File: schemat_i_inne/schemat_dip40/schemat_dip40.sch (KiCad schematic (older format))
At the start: 5 parts, among them J1 Conn_01x06_Female, U1 ATmega32A-PU, U2 Wincom_WG12864D-SFYLY, U3 SD_card_reader

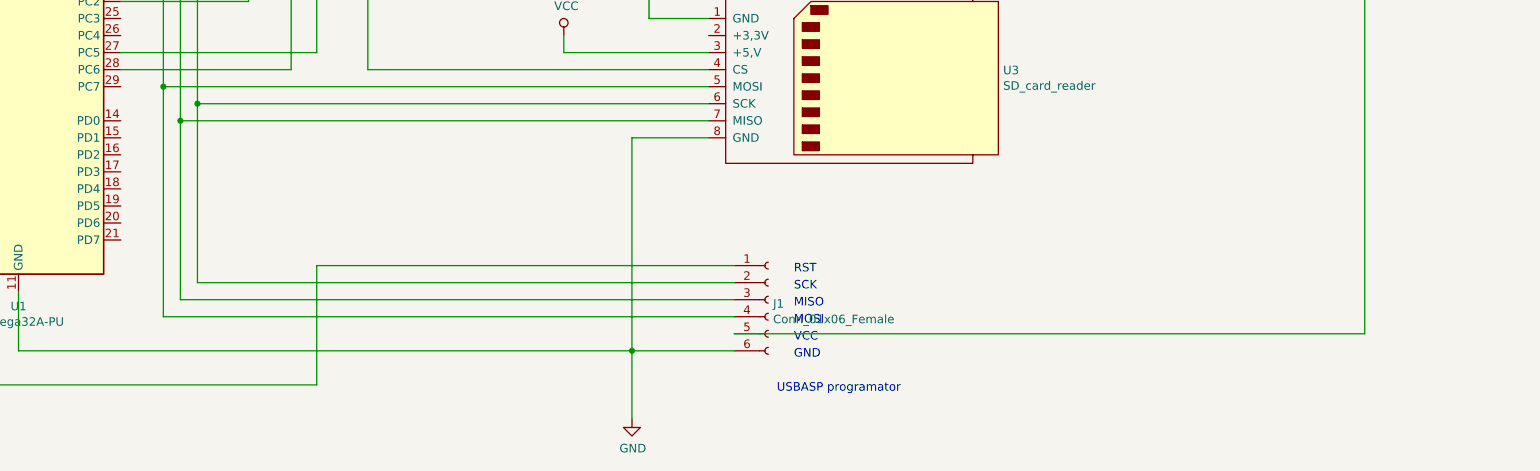
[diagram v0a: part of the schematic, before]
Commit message: Spaghetti dodane
Dodano przyciski do spaghetti układu
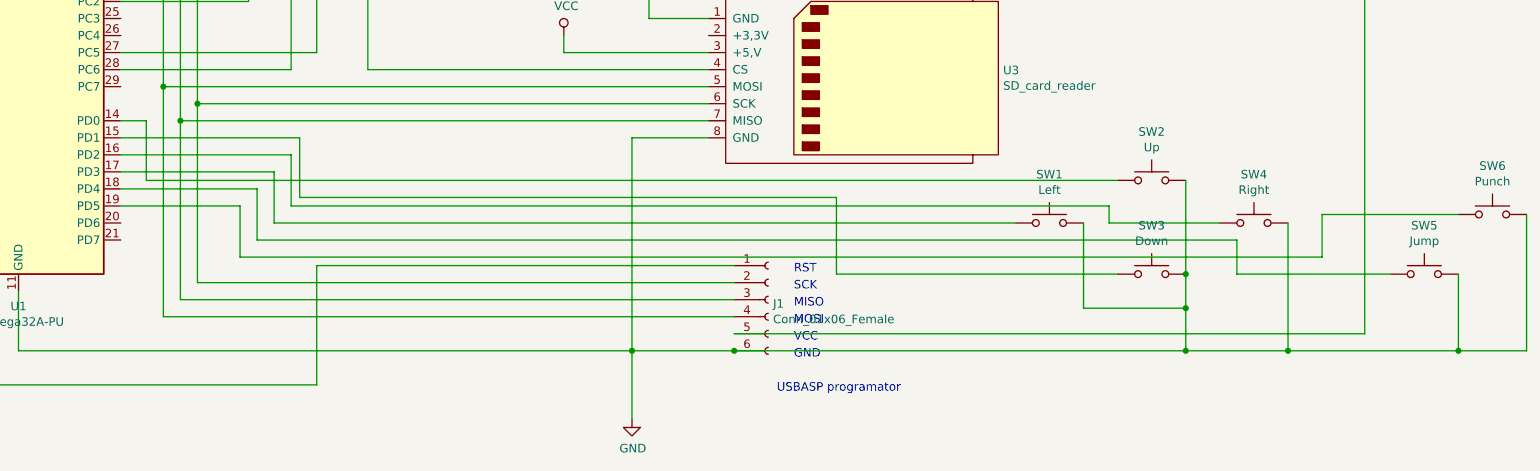
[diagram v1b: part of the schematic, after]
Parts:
- added SW1: Left, symbol Switch:SW_Push
- added SW2: Up, symbol Switch:SW_Push
- added SW3: Down, symbol Switch:SW_Push
- added SW4: Right, symbol Switch:SW_Push
- added SW5: Jump, symbol Switch:SW_Push
- added SW6: Punch, symbol Switch:SW_Push
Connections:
- net GND: now also SW1.2, SW2.2, SW3.2, SW4.2, SW5.2, SW6.2
- net at U1.14 (PD0): now also SW2.1
- net at U1.15 (PD1): now also SW3.1
- net at U1.16 (PD2): now also SW4.1
- net at U1.17 (PD3): now also SW1.1
- net at U1.18 (PD4): now also SW5.1
- net at U1.19 (PD5): now also SW6.1
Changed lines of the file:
@@
 $EndDescr
-$Comp
-L MCU_Microchip_ATmega:ATmega32A-PU U1
-U 1 1 61D4C9CD
-P 2250 3250
-F 0 "U1" H 2250 1161 50  0000 C CNN
-F 1 "ATmega32A-PU" H 2250 1070 50  0000 C CNN
-F 2 "Package_DIP:DIP-40_W15.24mm" H 2250 3250 50  0001 C CIN
-F 3 "http://ww1.microchip.com/downloads/en/DeviceDoc/atmel-8155-8-bit-microcontroller-avr-atmega32a_datasheet.pdf" H 2250 3250 50  0001 C CNN
-	1    2250 3250
-	1    0    0    -1
-$EndComp
 $Comp
 L schemat_dip40-rescue:Wincom_WG12864D-SFYLY-Display_Graphic U2
@@
 	5550 2150 5550 1550
 Wire Wire Line
-	5550 1550 2850 1550
-Wire Wire Line
 	6100 2250 5450 2250
 Wire Wire Line
 	5450 2250 5450 1650
 Wire Wire Line
-	5450 1650 2850 1650
-Wire Wire Line
 	6100 2350 5350 2350
 Wire Wire Line
 	5350 2350 5350 1750
 Wire Wire Line
-	5350 1750 2850 1750
-Wire Wire Line
 	6100 2450 5250 2450
 Wire Wire Line
 	5250 2450 5250 1850
 Wire Wire Line
-	5250 1850 2850 1850
-Wire Wire Line
 	6100 2550 5150 2550
 Wire Wire Line
 	5150 2550 5150 1950
 Wire Wire Line
-	5150 1950 2850 1950
-Wire Wire Line
 	6100 2650 5050 2650
 Wire Wire Line
 	5050 2650 5050 2050
 Wire Wire Line
-	5050 2050 2850 2050
-Wire Wire Line
 	6100 2750 4950 2750
 Wire Wire Line
 	4950 2750 4950 2150
 Wire Wire Line
-	4950 2150 2850 2150
-Wire Wire Line
 	6100 2850 4850 2850
 Wire Wire Line
 	4850 2850 4850 2250
 Wire Wire Line
-	4850 2250 2850 2250
-Wire Wire Line
 	6100 1650 5950 1650
 Wire Wire Line
@@
 	3500 1200 3500 3350
 Wire Wire Line
-	3500 3350 2850 3350
-Wire Wire Line
 	6100 1750 5850 1750
 Wire Wire Line
@@
 Wire Wire Line
 	3600 1300 3600 3550
-Wire Wire Line
-	3600 3550 2850 3550
 $Comp
 L power:VCC #PWR04
@@
 	3700 1450 3700 3450
 Wire Wire Line
-	3700 3450 2850 3450
-Wire Wire Line
 	6600 3050 6600 3200
 Wire Wire Line
@@
 	3850 3300 3850 3950
 Wire Wire Line
-	3850 3950 2850 3950
-Wire Wire Line
 	7100 2850 7400 2850
 Wire Wire Line
@@
 Wire Wire Line
 	4000 3400 4000 3850
-Wire Wire Line
-	4000 3850 2850 3850
 Wire Wire Line
 	7100 2350 7600 2350
@@
 $EndComp
 Wire Wire Line
-	2250 1250 2250 900
-Wire Wire Line
-	2350 1250 2350 900
-Wire Wire Line
 	2350 900  2250 900
 Connection ~ 2250 900
-Wire Wire Line
-	2250 5250 2250 5600
 Wire Wire Line
 	2250 5600 5850 5600
@@
 	1350 5800 1350 1550
 Wire Wire Line
-	1350 1550 1650 1550
-Wire Wire Line
 	6450 5200 3300 5200
 Wire Wire Line
 	3300 5200 3300 4150
 Wire Wire Line
-	3300 3150 2850 3150
-Wire Wire Line
 	6450 5300 3200 5300
 Wire Wire Line
 	3200 5300 3200 4250
 Wire Wire Line
-	3200 3050 2850 3050
-Wire Wire Line
 	6450 5400 3100 5400
 Wire Wire Line
 	3100 5400 3100 4050
 Wire Wire Line
-	3100 2950 2850 2950
-Wire Wire Line
 	6300 3950 4300 3950
 Wire Wire Line
 	4300 3950 4300 2650
-Wire Wire Line
-	4300 2650 2850 2650
 Wire Wire Line
 	6300 4050 3100 4050
@@
 	10150 5500 10150 2550
 Connection ~ 10150 2550
+$Comp
+L Switch:SW_Push SW2
+U 1 1 6261EEBB
+P 8900 4600
+F 0 "SW2" H 8900 4885 50  0000 C CNN
+F 1 "Up" H 8900 4794 50  0000 C CNN
+F 2 "" H 8900 4800 50  0001 C CNN
+F 3 "~" H 8900 4800 50  0001 C CNN
+	1    8900 4600
+	1    0    0    -1
+$EndComp
+$Comp
+L Switch:SW_Push SW3
+U 1 1 6261FEC3
+P 8900 5150
+F 0 "SW3" H 8900 5435 50  0000 C CNN
+F 1 "Down" H 8900 5344 50  0000 C CNN
+F 2 "" H 8900 5350 50  0001 C CNN
+F 3 "~" H 8900 5350 50  0001 C CNN
+	1    8900 5150
+	1    0    0    -1
+$EndComp
+$Comp
+L Switch:SW_Push SW4
+U 1 1 6262059D
+P 9500 4850
+F 0 "SW4" H 9500 5135 50  0000 C CNN
+F 1 "Right" H 9500 5044 50  0000 C CNN
+F 2 "" H 9500 5050 50  0001 C CNN
+F 3 "~" H 9500 5050 50  0001 C CNN
+	1    9500 4850
+	1    0    0    -1
+$EndComp
+$Comp
+L Switch:SW_Push SW1
+U 1 1 62620D64
+P 8300 4850
+F 0 "SW1" H 8300 5135 50  0000 C CNN
+F 1 "Left" H 8300 5044 50  0000 C CNN
+F 2 "" H 8300 5050 50  0001 C CNN
+F 3 "~" H 8300 5050 50  0001 C CNN
+	1    8300 4850
+	1    0    0    -1
+$EndComp
+$Comp
+L Switch:SW_Push SW5
+U 1 1 626213AA
+P 10500 5150
+F 0 "SW5" H 10500 5435 50  0000 C CNN
+F 1 "Jump" H 10500 5344 50  0000 C CNN
+F 2 "" H 10500 5350 50  0001 C CNN
+F 3 "~" H 10500 5350 50  0001 C CNN
+	1    10500 5150
+	1    0    0    -1
+$EndComp
+$Comp
+L Switch:SW_Push SW6
+U 1 1 6262299A
+P 10900 4800
+F 0 "SW6" H 10900 5085 50  0000 C CNN
+F 1 "Punch" H 10900 4994 50  0000 C CNN
+F 2 "" H 10900 5000 50  0001 C CNN
+F 3 "~" H 10900 5000 50  0001 C CNN
+	1    10900 4800
+	1    0    0    -1
+$EndComp
+Wire Wire Line
+	1350 1550 1650 1550
+Wire Wire Line
+	3300 3150 2850 3150
+Wire Wire Line
+	3200 3050 2850 3050
+Wire Wire Line
+	3100 2950 2850 2950
+Wire Wire Line
+	5550 1550 2850 1550
+Wire Wire Line
+	5450 1650 2850 1650
+Wire Wire Line
+	5350 1750 2850 1750
+Wire Wire Line
+	5250 1850 2850 1850
+Wire Wire Line
+	5150 1950 2850 1950
+Wire Wire Line
+	5050 2050 2850 2050
+Wire Wire Line
+	4950 2150 2850 2150
+Wire Wire Line
+	4850 2250 2850 2250
+Wire Wire Line
+	2350 1250 2350 900
+Wire Wire Line
+	4300 2650 2850 2650
+Wire Wire Line
+	3850 3950 2850 3950
+Wire Wire Line
+	4000 3850 2850 3850
+Wire Wire Line
+	3600 3550 2850 3550
+Wire Wire Line
+	3700 3450 2850 3450
+Wire Wire Line
+	3500 3350 2850 3350
+Wire Wire Line
+	2250 5250 2250 5600
+Wire Wire Line
+	2250 1250 2250 900
+$Comp
+L MCU_Microchip_ATmega:ATmega32A-PU U1
+U 1 1 61D4C9CD
+P 2250 3250
+F 0 "U1" H 2250 1161 50  0000 C CNN
+F 1 "ATmega32A-PU" H 2250 1070 50  0000 C CNN
+F 2 "Package_DIP:DIP-40_W15.24mm" H 2250 3250 50  0001 C CIN
+F 3 "http://ww1.microchip.com/downloads/en/DeviceDoc/atmel-8155-8-bit-microcontroller-avr-atmega32a_datasheet.pdf" H 2250 3250 50  0001 C CNN
+	1    2250 3250
+	1    0    0    -1
+$EndComp
+Wire Wire Line
+	8700 4600 3000 4600
+Wire Wire Line
+	3000 4600 3000 4250
+Wire Wire Line
+	3000 4250 2850 4250
+Wire Wire Line
+	8700 5150 7050 5150
+Wire Wire Line
+	7050 5150 7050 4700
+Wire Wire Line
+	7050 4700 3900 4700
+Wire Wire Line
+	3900 4700 3900 4350
+Wire Wire Line
+	3900 4350 2850 4350
+Wire Wire Line
+	9300 4850 8650 4850
+Wire Wire Line
+	8650 4850 8650 4750
+Wire Wire Line
+	8650 4750 3850 4750
+Wire Wire Line
+	3850 4750 3850 4450
+Wire Wire Line
+	3850 4450 2850 4450
+Wire Wire Line
+	8100 4850 3750 4850
+Wire Wire Line
+	3750 4850 3750 4550
+Wire Wire Line
+	3750 4550 2850 4550
+Wire Wire Line
+	10300 5150 9400 5150
+Wire Wire Line
+	9400 5150 9400 4950
+Wire Wire Line
+	9400 4950 3650 4950
+Wire Wire Line
+	3650 4950 3650 4650
+Wire Wire Line
+	3650 4650 2850 4650
+Wire Wire Line
+	10700 4800 9900 4800
+Wire Wire Line
+	9900 4800 9900 5050
+Wire Wire Line
+	9900 5050 3550 5050
+Wire Wire Line
+	3550 5050 3550 4750
+Wire Wire Line
+	3550 4750 2850 4750
+Wire Wire Line
+	6450 5600 9100 5600
+Wire Wire Line
+	9100 5600 9100 5350
+Connection ~ 6450 5600
+Wire Wire Line
+	9100 5600 9700 5600
+Wire Wire Line
+	9700 5600 9700 4850
+Connection ~ 9100 5600
+Wire Wire Line
+	9700 5600 10700 5600
+Wire Wire Line
+	10700 5600 10700 5150
+Connection ~ 9700 5600
+Wire Wire Line
+	10700 5600 11100 5600
+Wire Wire Line
+	11100 5600 11100 4800
+Connection ~ 10700 5600
+Wire Wire Line
+	9100 5150 9100 4600
+Connection ~ 9100 5150
+Wire Wire Line
+	9100 5350 8500 5350
+Wire Wire Line
+	8500 5350 8500 4850
+Connection ~ 9100 5350
+Wire Wire Line
+	9100 5350 9100 5150
 $EndSCHEMATC
